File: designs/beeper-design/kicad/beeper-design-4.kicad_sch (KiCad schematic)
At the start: 23 parts, among them U13 CSD75207W15, U3 BQ51003YFPR

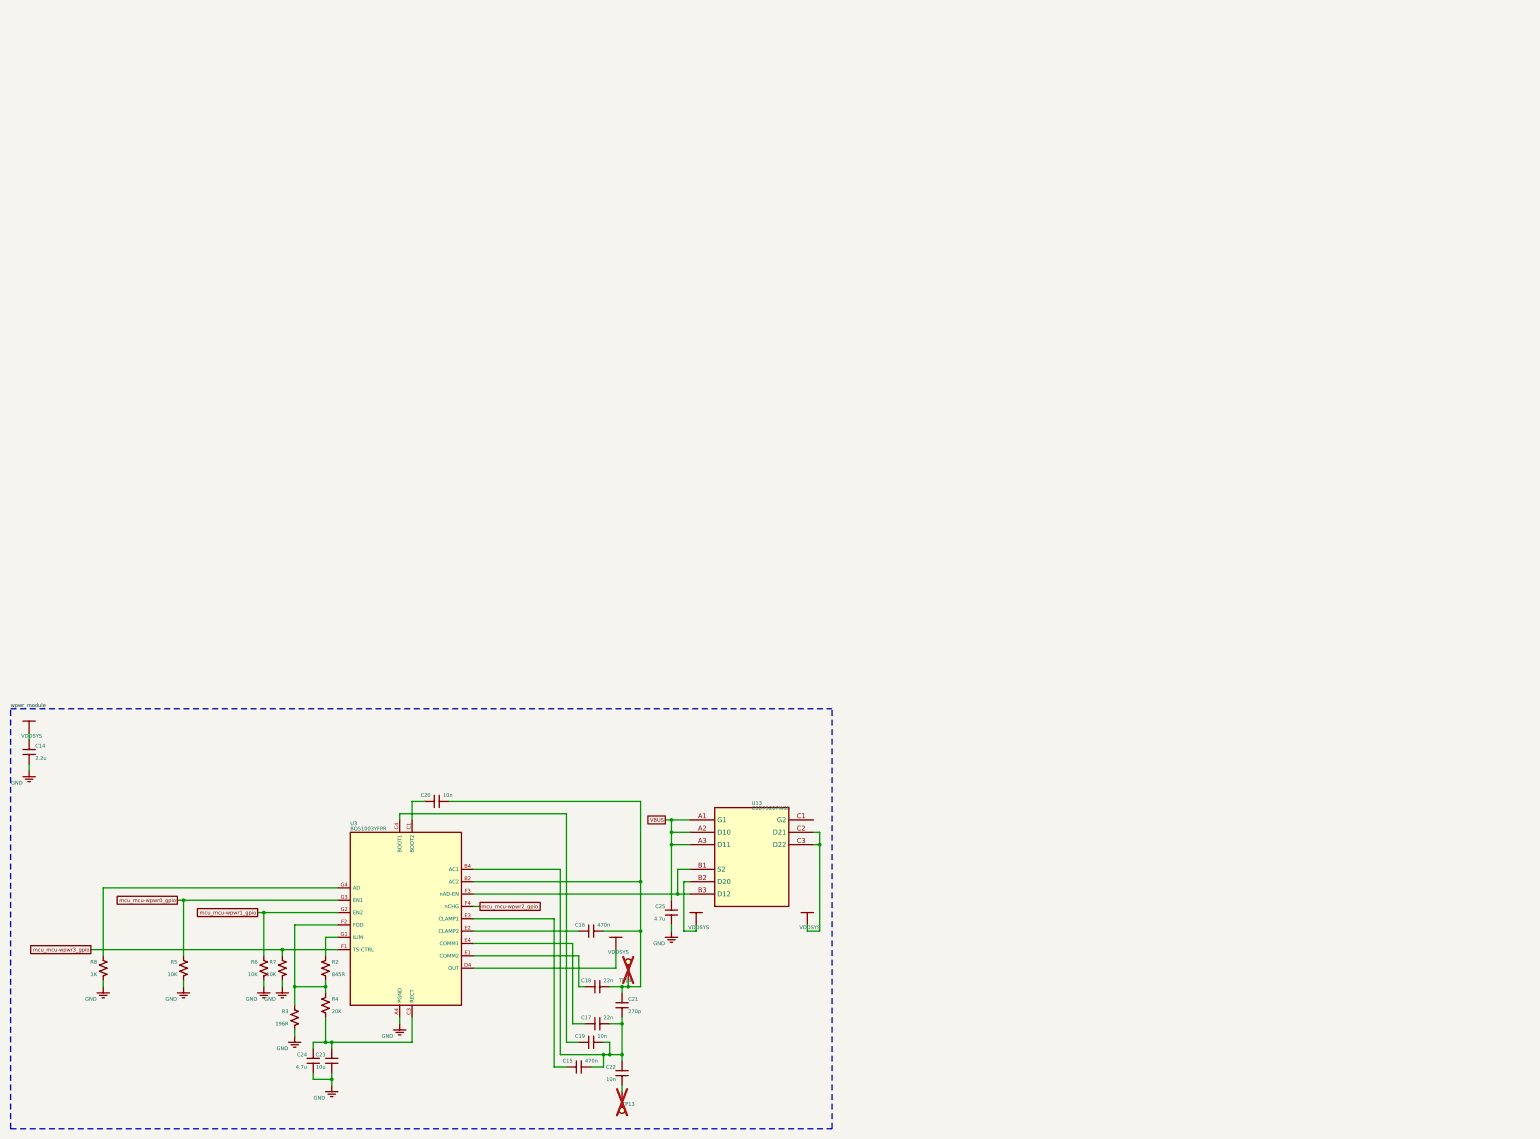
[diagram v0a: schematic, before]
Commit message: post export, had to munge sch
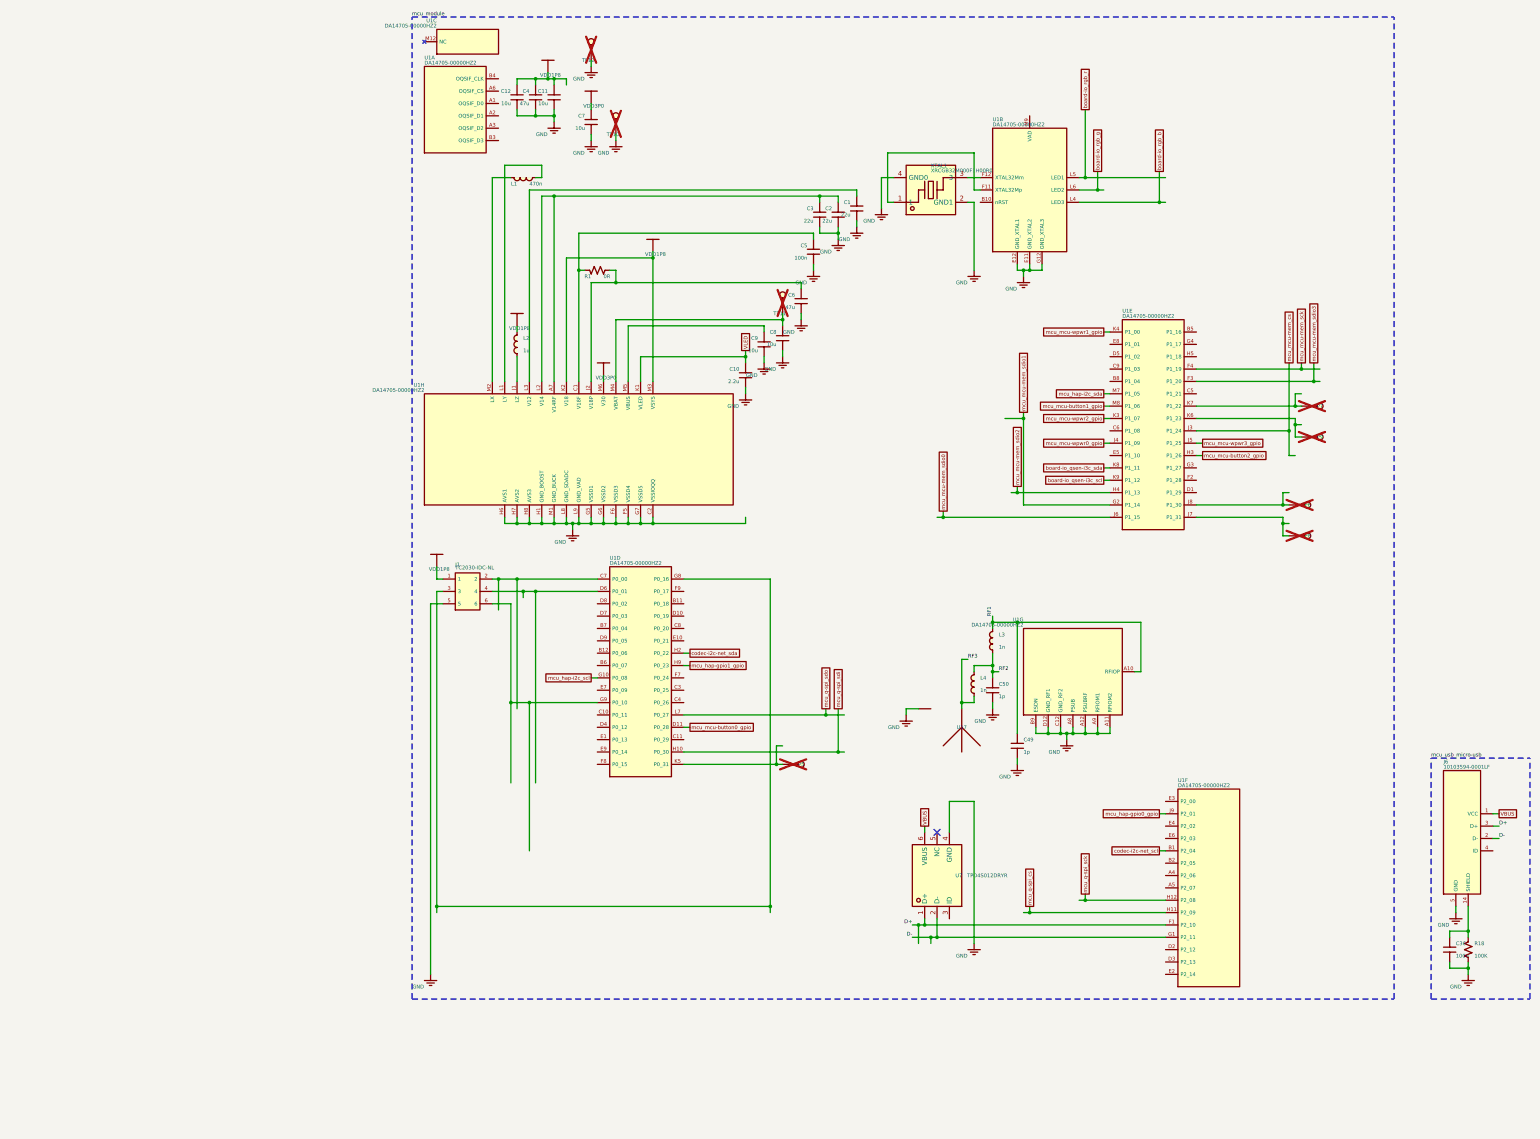
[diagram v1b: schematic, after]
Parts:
- removed C14: 2.2u, beeper-design:Pkg0201_41, symbol C318539_1
- removed C15: 470n, beeper-design:Pkg0402_5, symbol C106255
- removed C16: 470n, beeper-design:Pkg0402_10, symbol C106255_1
- removed C17: 22n, beeper-design:Pkg0201_14, symbol my_capacitor_2
- removed C18: 22n, beeper-design:Pkg0201_26, symbol my_capacitor_4
- removed C19: 10n, beeper-design:Pkg0201_36, symbol C272853_1
- removed C20: 10n, beeper-design:Pkg0201_45, symbol C272853_2
- removed C21: 270p, beeper-design:Pkg0201_12, symbol my_capacitor
- removed C22: 10n, beeper-design:Pkg0201_23, symbol C272853
- removed C23: 10u, beeper-design:Pkg0402_3, symbol C962143_3
- removed C24: 4.7u, beeper-design:Pkg0402_8, symbol C386043_1
- removed C25: 4.7u, beeper-design:Pkg0402_6, symbol C386043
- removed R2: 845R, beeper-design:Pkg0201_6, symbol my_resistor_1
- removed R3: 196R, beeper-design:Pkg0201_17, symbol C138167
- removed R4: 20K, beeper-design:Pkg0201_29, symbol C295787
- removed R5: 10K, beeper-design:Pkg0201_39, symbol C138117_1
- removed R6: 10K, beeper-design:Pkg0201_4, symbol C138117_2
- removed R7: 10K, beeper-design:Pkg0201_16, symbol C138117
- removed R8: 1K, beeper-design:Pkg0201_28, symbol C131396
- removed TP13, TP14: (no value), beeper-design:SMD_TESTPT, symbol smd_testpoint_cmp
- removed U13: CSD75207W15, beeper-design:LP_6, symbol CSD75207W15
- removed U3: BQ51003YFPR, beeper-design:LP_7, symbol BQ51003YFPR
- added C1: 22u, beeper-design:Pkg0603_2, symbol my_capacitor_12
- added C10: 2.2u, beeper-design:Pkg0201_42, symbol my_capacitor_15
- added C11: 10u, beeper-design:Pkg0402_8, symbol C105225_5
- added C12: 10u, beeper-design:Pkg0402, symbol C105225
- added C2: 22u, beeper-design:Pkg0603, symbol my_capacitor_19
- added C3: 22u, beeper-design:Pkg0603_1, symbol my_capacitor_3
- added C36: 100n, beeper-design:Pkg0201_8, symbol my_capacitor_1
- added C4: 47u, beeper-design:Pkg0805, symbol my_capacitor_6
- added C49: 1p, beeper-design:Pkg0201_16, symbol C161376
- added C5: 100n, beeper-design:Pkg0201_32, symbol my_capacitor_11
- added C50: 1p, beeper-design:Pkg0201_33, symbol C161376_1
- added C6: 47u, beeper-design:Pkg0805_1, symbol my_capacitor_17
- added C7: 10u, beeper-design:Pkg0402_1, symbol C105225_1
- added C8: 10u, beeper-design:Pkg0402_3, symbol C105225_3
- added C9: 10u, beeper-design:Pkg0402_7, symbol C105225_4
- added J1: TC2030-IDC-NL, beeper-design:TC2030_IDC_NL_FOOTPRINT, symbol component
- added J6: 10103594-0001LF, beeper-design:AMPHENOL_10103594_0001LF, symbol AMPHENOL_10103594_0001LF
- added L1: 470n, beeper-design:Pkg0201_14, symbol my_inductor
- added L2: 1u, beeper-design:Pkg0402_5, symbol C516791
- added L3: 1n, beeper-design:Pkg0201_24, symbol my_inductor_1
- added L4: 1n, beeper-design:Pkg0201_41, symbol my_inductor_2
- added R1: 0R, beeper-design:Pkg0201_4, symbol my_resistor_1
- added R18: 100K, beeper-design:Pkg0201_44, symbol my_resistor_11
- added TP10, TP11, TP12, TP5, TP6, TP7, TP8, TP9: (no value), beeper-design:SMD_TESTPT, symbol smd_testpoint_cmp
- added U1: DA14705-00000HZ2, beeper-design:LP, symbol DA14705
- added U17: (no value), beeper-design:Pkg_2450AT18D0100_STD_R_1, symbol Sym2450AT18D0100
- added U7: TPD4S012DRYR, beeper-design:SON_6_L1_5_W1_0_P0_50_BL, symbol C96506
- added XTAL1: XRCGB32M000F1H00R0, beeper-design:CRYSTAL_SMD_4P_L2_0_W1_6_BL_1, symbol C880116
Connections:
- net GND: now also C1.1, C10.1, C11.1, C12.1, C2.1, C3.1, C36.2, C4.1, C49.2, C5.1, C50.2, C6.1, C7.1, C8.1, C9.1, J1.5, J6.5 (GND), R18.2, TP10.p, TP12.p, U1.A11 (RFIOM2), U1.A12 (PSUBRF), U1.A8 (PSUB), U1.A9 (RFIOM1), U1.B9 (ESDN), U1.C12 (GND_RF2), U1.C2 (VSSIOQQ), U1.D12 (GND_RF1), U1.E11 (GND_XTAL2), U1.E12 (GND_XTAL1), U1.F5 (VSSD4), U1.F6 (VSSD3), U1.G12 (GND_XTAL3), U1.G5 (VSSD1), U1.G6 (VSSD2), U1.G7 (VSSD5), U1.H1 (GND_BOOST), U1.H6 (AVS1), U1.H7 (AVS2), U1.H8 (AVS3), U1.L8 (GND_SDADC), U1.L9 (GND_VAD), U1.M1 (GND_BUCK), U17.2 (GND), U17.3 (GND), U17.4 (GND), U7.4 (GND), XTAL1.2 (GND1), XTAL1.4 (GND0)
- net VBUS: now also J6.1 (VCC), U7.6 (VBUS)
- net mcu_mcu-wpwr0_gpio: now also U1.J4 (P1_09)
- net mcu_mcu-wpwr1_gpio: now also U1.K4 (P1_00)
- net mcu_mcu-wpwr2_gpio: now also U1.K3 (P1_07)
- net mcu_mcu-wpwr3_gpio: now also U1.J5 (P1_25)
- new net: L1.1, U1.M2 (LX)
- new net: L1.2, U1.L1 (LY)
- new net: C6.2, R1.2, U1.J2 (V18P)
- new net: C9.2, U1.M5 (VBUS)
- new net: J1.2, U1.C7 (P0_00)
- new net: J1.4, U1.D6 (P0_01)
- new net: J1.3, U1.G8 (P0_16)
- new net: J1.6, U1.G9 (P0_10)
- new net: TP5.p, U1.K5 (P0_31)
- new net: C5.2, R1.1, U1.C1 (V18F)
- new net: C2.2, C3.2, U1.A7 (V14RF), U1.L2 (V14)
- new net: U1.F11 (XTAL32Mp), XTAL1.1
- new net: U1.F12 (XTAL32Mm), XTAL1.3
- new net: C36.1, J6.10 (SHIELD), J6.11 (SHIELD), J6.13 (SHIELD), J6.14 (SHIELD), J6.6 (SHIELD), J6.7 (SHIELD), J6.8 (SHIELD), J6.9 (SHIELD), R18.1
- new net: L2.1, U1.J1 (LZ)
- new net: C1.2, U1.L3 (V12)
- new net: C8.2, TP11.p, U1.M4 (VBAT)
- new net: TP7.p, U1.K7 (P1_22)
- new net: TP8.p, U1.J7 (P1_31)
- new net: TP6.p, U1.J8 (P1_30)
- new net: TP9.p, U1.K6 (P1_23)
- new net: U1.J10 (NC), U1.J11 (NC), U1.J12 (NC), U1.K10 (NC), U1.K11 (NC), U1.K12 (NC), U1.L10 (NC), U1.L11 (NC), U1.L12 (NC), U1.M10 (NC), U1.M11 (NC), U1.M12 (NC)
- new net D+: J6.3 (D+), U1.F1 (P2_10), U7.1 (D+)
- new net D-: J6.2 (D-), U1.G1 (P2_11), U7.2 (D-)
- new net RF1: C49.1, L3.1, U1.A10 (RFIOP)
- new net RF2: C50.1, L3.2, L4.1
- new net RF3: L4.2, U17.1 (ANT)
- new net VDD1P8: C11.2, C12.2, C4.2, J1.1, L2.2, U1.K2 (V18), U1.M3 (VSYS)
- new net VDD3P0: C7.2, U1.M6 (V30)
- new net VLED: C10.2, U1.K1 (VLED)
- new net board-io_qsen-i3c_scl: U1.K9 (P1_12)
- new net board-io_qsen-i3c_sda: U1.K8 (P1_11)
- new net board-io_rgb_b: U1.L4 (LED3)
- new net board-io_rgb_g: U1.L6 (LED2)
- new net board-io_rgb_r: U1.L5 (LED1)
- new net codec-i2c-net_scl: U1.B1 (P2_04)
- new net codec-i2c-net_sda: U1.H2 (P0_22)
- new net mcu_hap-gpio0_gpio: U1.J9 (P2_01)
- new net mcu_hap-gpio1_gpio: U1.H9 (P0_23)
- new net mcu_hap-i2c_scl: U1.G10 (P0_08)
- new net mcu_hap-i2c_sda: U1.M7 (P1_05)
- new net mcu_mcu-button0_gpio: U1.D11 (P0_28)
- new net mcu_mcu-button1_gpio: U1.M8 (P1_06)
- new net mcu_mcu-button2_gpio: U1.H3 (P1_26)
- new net mcu_mcu-mem_cs: U1.J3 (P1_24)
- new net mcu_mcu-mem_sck: U1.F4 (P1_19)
- new net mcu_mcu-mem_sdio0: U1.J6 (P1_15)
- new net mcu_mcu-mem_sdio1: U1.G2 (P1_14)
- new net mcu_mcu-mem_sdio2: U1.H4 (P1_13)
- new net mcu_mcu-mem_sdio3: U1.F3 (P1_20)
- new net mcu_q-spi_cs: U1.H11 (P2_09)
- new net mcu_q-spi_sck: U1.H12 (P2_08)
- new net mcu_q-spi_sdi: U1.H10 (P0_30)
- new net mcu_q-spi_sdo: U1.L7 (P0_27)
- no-connect marks 0 -> 1
